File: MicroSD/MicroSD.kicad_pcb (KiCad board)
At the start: 2 copper layers, 25.4 x 28.6 mm, 17 parts, among them J1 Conn_01x08, U1 AP7365, U2 4050

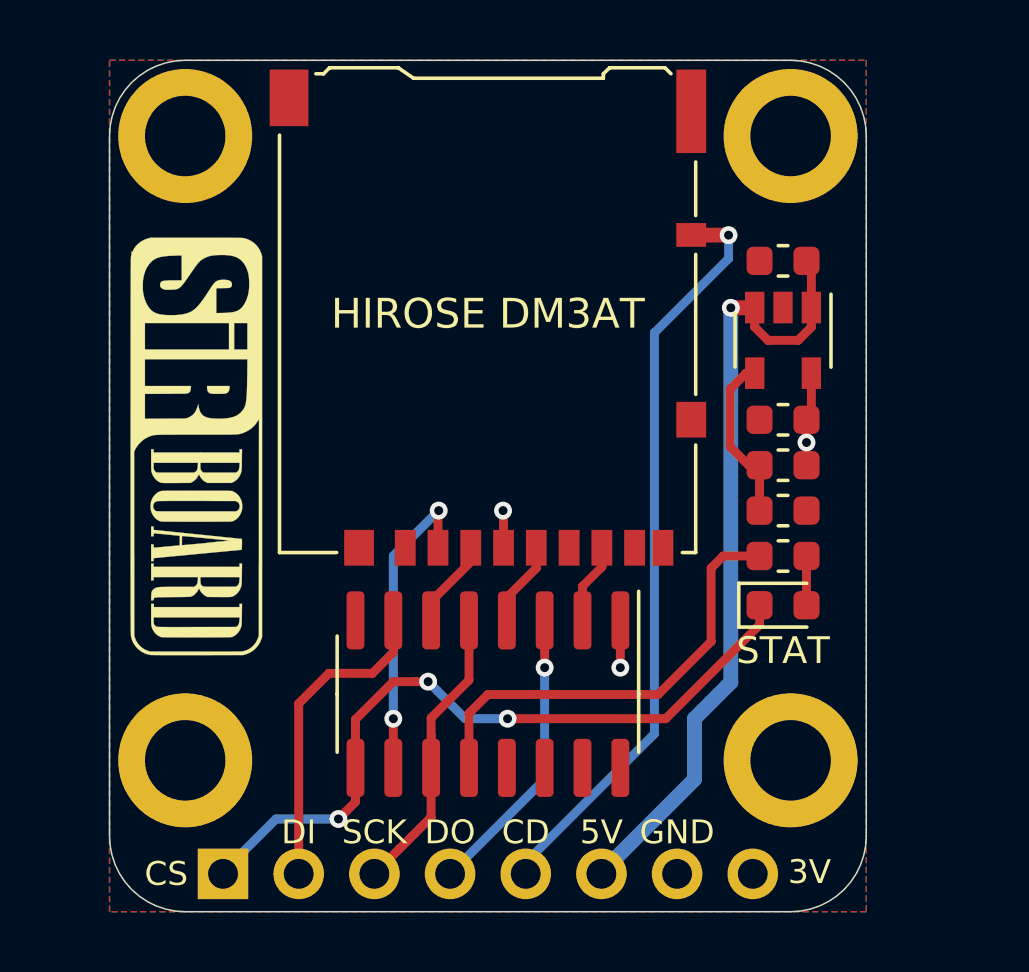
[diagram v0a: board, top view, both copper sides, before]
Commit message: Board Redesign
Revision3
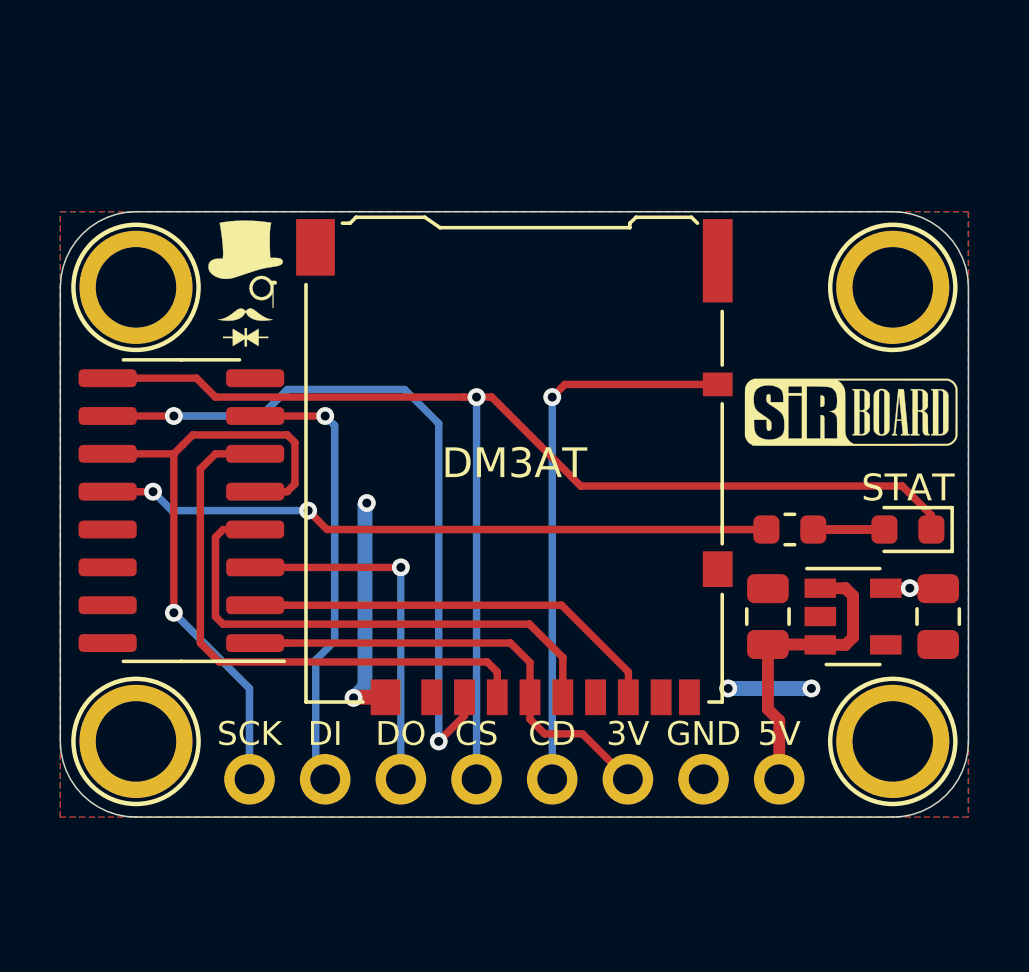
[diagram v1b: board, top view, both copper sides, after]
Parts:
- removed R1: 31K6, Resistor_SMD:R_0603_1608Metric
- removed R3: 10K, Resistor_SMD:R_0603_1608Metric
- added G***: LOGO, logo:logo42x59, F.Cu at (56.3, 26.3)
- C1, C2: value 1uF -> 10uF; footprint Capacitor_SMD:C_0603_1608Metric -> Capacitor_SMD:C_0805_2012Metric
- DM3AT: renamed from HIROSE DM3AT
- G***: footprint logo:logo126x178 -> logo:logo76x107
- G***: footprint logo:SirBoard140x44 -> logo:SirBoard112x35
- G***: footprint logo:SirBoard140x44 -> logo:SirBoard71X22
- H1, H2, H3, H4: footprint MountingHole:MountingHole_2.7mm_M2.5_ISO14580_Pad -> SirBoardLibrary:MountingHole_M2.5_SirBoard
- U1: value AP7365 -> AP2127K-3.3
- moved H2 23.8 mm to (78.0, 41.7), turned to 90 degrees
- moved H3 22.6 mm to (52.6, 26.4), turned to 90 degrees
- moved G*** 22.0 mm to (76.6, 30.6), turned to 0 degrees
- moved H1 20.4 mm to (52.6, 41.7), turned to 90 degrees
- moved H4 16.2 mm to (78.0, 26.4), turned to 90 degrees
- moved U2 12.0 mm to (54.1, 33.9), turned to 180 degrees
- moved C1 11.9 mm to (73.8, 37.5), turned to 90 degrees
- moved U1 9.56 mm to (76.6, 37.5), turned to 0 degrees
- moved C2 8.41 mm to (79.5, 37.5), turned to 270 degrees
- moved DM3AT 5.09 mm to (65.3, 32.4)
- moved STAT 4.90 mm to (78.5, 34.5), turned to 180 degrees
- moved J1 3.30 mm to (56.4, 42.9)
- moved G*** 2.57 mm to (65.3, 28.1)
- moved G*** 0.97 mm to (65.3, 34.0)
- moved R6 0.92 mm to (74.5, 34.5)
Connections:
- J1 pad 1: CS -> SCK
- J1 pad 3: SCK -> DO
- J1 pad 4: DO -> CS
- J1 pad 6: VIN -> VOUT
- J1 pad 8: VOUT -> VIN
- U1 pad 4: ADJ -> Net-(U1-Pad4)
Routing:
- net CS: track 24.8 -> 42.9 mm, vias 3 -> 1
- net VIN: track 26.8 -> 10.3 mm, vias 1 -> 0
- net /DI_SD: track 2.99 -> 19.1 mm
- net /CLK_SD: track 2.85 -> 17.7 mm
- net /CS_SD: track 10.5 -> 24.5 mm
- net SCK: track 9.82 -> 21.5 mm, vias 0 -> 1
- net /DO_SD: track 2.71 -> 14.3 mm
- net VOUT: track 6.00 -> 17.3 mm, vias 3 -> 1
- net GND: track 0.00 -> 10.6 mm, vias 0 -> 4
- net Net-(R6-Pad1): track 15.2 -> 22.6 mm, vias 0 -> 2
- net DETA: track 25.5 -> 18.6 mm
- net ADJ: track 5.75 -> 0.00 mm
- net DI: track 10.7 -> 15.1 mm, vias 0 -> 1
- net DO: track 9.82 -> 12.0 mm
- net Net-(D1-Pad2): track 1.65 -> 2.39 mm
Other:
- board size 25.4 x 28.6 mm -> 30.5 x 20.3 mm
- board text added: "MicroSD to DIP Breakout With 74HC4050 Level-Shift"
- board text removed: "MicroSD to DIP Breakout 74HC4050 Level-Shift"
